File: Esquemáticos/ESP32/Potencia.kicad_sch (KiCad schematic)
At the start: 12 parts, among them J3 Barrel_Jack, SW1 SW_DIP_x01, U5 AMS1117-5.0, U6 AMS1117-3.3

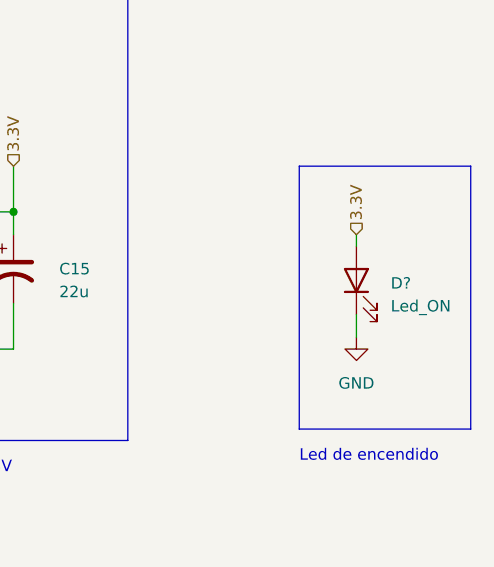
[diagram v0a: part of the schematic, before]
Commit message: Asignación Huellas de Resistencias
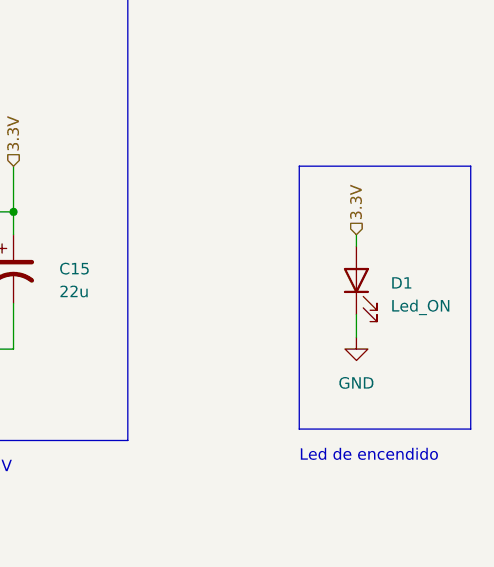
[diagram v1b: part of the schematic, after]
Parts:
- SW1: footprint (none) -> Button_Switch_SMD:SW_DIP_SPSTx01_Slide_6.7x4.1mm_W6.73mm_P2.54mm_LowProfile_JPin
- gave numbers to parts that had none: 1
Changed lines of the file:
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@@
   (symbol (lib_id "LED:IR26-21C_L110_TR8") (at 245.11 135.89 90) (unit 1)
     (in_bom yes) (on_board yes) (fields_autoplaced)
-    (property "Reference" "D?" (id 0) (at 248.92 136.2074 90)
+    (property "Reference" "D1" (id 0) (at 248.92 136.2074 90)
       (effects (font (size 1.27 1.27)) (justify right))
     )
@@
   (symbol (lib_id "power:GND") (at 245.11 142.24 0) (unit 1)
     (in_bom yes) (on_board yes) (fields_autoplaced)
-    (property "Reference" "#PWR?" (id 0) (at 245.11 148.59 0)
+    (property "Reference" "#PWR0101" (id 0) (at 245.11 148.59 0)
       (effects (font (size 1.27 1.27)) hide)
     )
@@
     (property "Reference" "SW1" (id 0) (at 88.9 81.28 0))
     (property "Value" "SW_DIP_x01" (id 1) (at 88.9 83.82 0))
-    (property "Footprint" "" (id 2) (at 88.9 88.9 0)
+    (property "Footprint" "Button_Switch_SMD:SW_DIP_SPSTx01_Slide_6.7x4.1mm_W6.73mm_P2.54mm_LowProfile_JPin" (id 2) (at 88.9 88.9 0)
       (effects (font (size 1.27 1.27)) hide)
     )

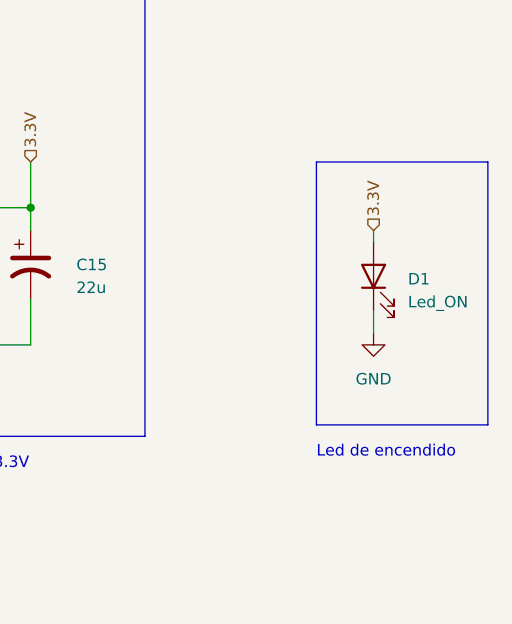
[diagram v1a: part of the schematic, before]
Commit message: lol
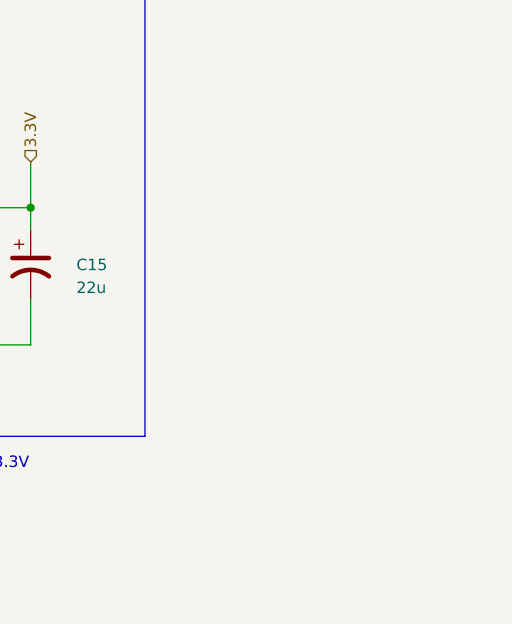
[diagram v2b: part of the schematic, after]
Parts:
- removed D1: Led_ON, LED_SMD:LED_1206_3216Metric, symbol LED:IR26-21C_L110_TR8
- SW1: footprint Button_Switch_SMD:SW_DIP_SPSTx01_Slide_6.7x4.1mm_W6.73mm_P2.54mm_LowProfile_JPin -> (none)
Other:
- note removed: "Led de encendido"
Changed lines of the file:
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@@
-    (stroke (width 0) (type default) (color 0 0 0 0))
-  )
-  (polyline (pts (xy 238.76 123.19) (xy 238.76 152.4))
     (stroke (width 0) (type default) (color 0 0 0 0))
   )
@@
     (stroke (width 0) (type default) (color 0 0 0 0))
   )
-  (polyline (pts (xy 257.81 152.4) (xy 257.81 123.19))
-    (stroke (width 0) (type default) (color 0 0 0 0))
-  )
   (wire (pts (xy 163.83 138.43) (xy 163.83 143.51))
     (stroke (width 0) (type default) (color 0 0 0 0))
@@
     (stroke (width 0) (type default) (color 0 0 0 0))
   )
-  (polyline (pts (xy 238.76 123.19) (xy 257.81 123.19))
-    (stroke (width 0) (type default) (color 0 0 0 0))
-  )
-  (wire (pts (xy 245.11 139.7) (xy 245.11 142.24))
-    (stroke (width 0) (type default) (color 0 0 0 0))
-  )
   (wire (pts (xy 207.01 91.44) (xy 207.01 88.9))
     (stroke (width 0) (type default) (color 0 0 0 0))
@@
     (stroke (width 0) (type default) (color 0 0 0 0))
   )
-  (wire (pts (xy 245.11 130.81) (xy 245.11 132.08))
-    (stroke (width 0) (type default) (color 0 0 0 0))
-  )
   (wire (pts (xy 163.83 120.65) (xy 163.83 128.27))
     (stroke (width 0) (type default) (color 0 0 0 0))
@@
     (stroke (width 0) (type default) (color 0 0 0 0))
   )
-  (polyline (pts (xy 238.76 152.4) (xy 257.81 152.4))
-    (stroke (width 0) (type default) (color 0 0 0 0))
-  )
   (wire (pts (xy 160.02 88.9) (xy 160.02 91.44))
     (stroke (width 0) (type default) (color 0 0 0 0))
@@
   )
   (text "Entrada de alimentación de 12V mediante un Jack " (at 76.2 123.19 0)
-    (effects (font (size 1.27 1.27)) (justify left bottom))
-  )
-  (text "Led de encendido\n" (at 238.76 156.21 0)
     (effects (font (size 1.27 1.27)) (justify left bottom))
   )
@@
   )
   (hierarchical_label "3.3V" (shape input) (at 207.01 123.19 90)
-    (effects (font (size 1.27 1.27)) (justify left))
-  )
-  (hierarchical_label "3.3V" (shape input) (at 245.11 130.81 90)
     (effects (font (size 1.27 1.27)) (justify left))
   )
@@
     (pin "1")
   )
-  (symbol (lib_id "LED:IR26-21C_L110_TR8") (at 245.11 135.89 90) (unit 1)
-    (in_bom yes) (on_board yes) (fields_autoplaced)
-    (property "Reference" "D1" (id 0) (at 248.92 136.2074 90)
-      (effects (font (size 1.27 1.27)) (justify right))
-    )
-    (property "Value" "Led_ON" (id 1) (at 248.92 138.7474 90)
-      (effects (font (size 1.27 1.27)) (justify right))
-    )
-    (property "Footprint" "LED_SMD:LED_1206_3216Metric" (id 2) (at 240.03 135.89 0)
-      (effects (font (size 1.27 1.27)) hide)
-    )
-    (property "Datasheet" "http://www.everlight.com/file/ProductFile/IR26-21C-L110-TR8.pdf" (id 3) (at 245.11 135.89 0)
-      (effects (font (size 1.27 1.27)) hide)
-    )
-    (pin "1")
-    (pin "2")
-  )
   (symbol (lib_id "Device:C_Polarized_US") (at 163.83 134.62 0) (unit 1)
     (in_bom yes) (on_board yes)
@@
     (pin "1")
   )
-  (symbol (lib_id "power:GND") (at 245.11 142.24 0) (unit 1)
-    (in_bom yes) (on_board yes) (fields_autoplaced)
-    (property "Reference" "#PWR0101" (id 0) (at 245.11 148.59 0)
-      (effects (font (size 1.27 1.27)) hide)
-    )
-    (property "Value" "GND" (id 1) (at 245.11 147.32 0))
-    (property "Footprint" "" (id 2) (at 245.11 142.24 0)
-      (effects (font (size 1.27 1.27)) hide)
-    )
-    (property "Datasheet" "" (id 3) (at 245.11 142.24 0)
-      (effects (font (size 1.27 1.27)) hide)
-    )
-    (pin "1")
-  )
   (symbol (lib_id "power:GND") (at 113.03 107.95 0) (unit 1)
     (in_bom yes) (on_board yes) (fields_autoplaced)
@@
     (property "Reference" "SW1" (id 0) (at 88.9 81.28 0))
     (property "Value" "SW_DIP_x01" (id 1) (at 88.9 83.82 0))
-    (property "Footprint" "Button_Switch_SMD:SW_DIP_SPSTx01_Slide_6.7x4.1mm_W6.73mm_P2.54mm_LowProfile_JPin" (id 2) (at 88.9 88.9 0)
-      (effects (font (size 1.27 1.27)) hide)
-    )
+    (property "Footprint" "" (id 2) (at 88.9 88.9 0)
+      (effects (font (size 1.27 1.27)) hide)
+    )
